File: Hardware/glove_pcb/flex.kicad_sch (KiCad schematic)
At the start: 9 parts

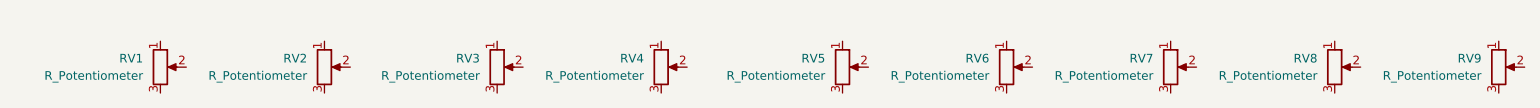
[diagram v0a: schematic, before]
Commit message: More work on motor driver connection
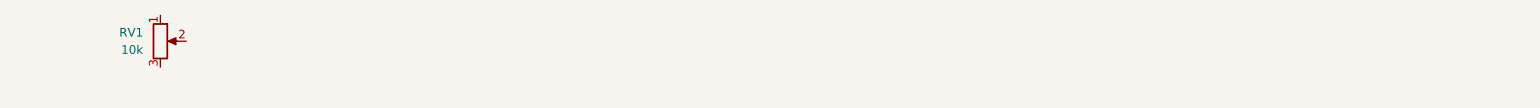
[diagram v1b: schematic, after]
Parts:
- removed RV2, RV3, RV4, RV5, RV6, RV7, RV8, RV9: R_Potentiometer, symbol Device:R_Potentiometer
- RV1: value R_Potentiometer -> 10k
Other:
- moved on the sheet: RV1
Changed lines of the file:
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@@
 (kicad_sch (version 20230121) (generator eeschema)
   (paper "A4")
-  (symbol (lib_id "Device:R_Potentiometer") (at 124.46 45.72 0) (unit 1)
+  (symbol (lib_id "Device:R_Potentiometer") (at 50.8 41.91 0) (unit 1)
     (in_bom yes) (on_board yes) (dnp no) (fields_autoplaced)
-    (property "Reference" "RV4" (at 121.92 44.45 0)
+    (property "Reference" "RV1" (at 48.26 40.64 0)
       (effects (font (size 1.27 1.27)) (justify right))
     )
-    (property "Value" "R_Potentiometer" (at 121.92 46.99 0)
+    (property "Value" "10k" (at 48.26 43.18 0)
       (effects (font (size 1.27 1.27)) (justify right))
     )
-    (property "Footprint" "" (at 124.46 45.72 0)
+    (property "Footprint" "" (at 50.8 41.91 0)
       (effects (font (size 1.27 1.27)) hide)
     )
-    (property "Datasheet" "~" (at 124.46 45.72 0)
-      (effects (font (size 1.27 1.27)) hide)
-    )
-    (pin "1")
-    (pin "2")
-    (pin "3")
-    (instances
-      (project "glove_pcb"
-        (path "/747ff5f3-d342-40b0-8e4e-75b3a3063e75"
-          (reference "RV4") (unit 1)
-        )
-        (path "/747ff5f3-d342-40b0-8e4e-75b3a3063e75/bbbc9975-a050-48bd-8c18-11f2eff17087"
-          (reference "RV4") (unit 1)
-        )
-      )
-    )
-  )
-  (symbol (lib_id "Device:R_Potentiometer") (at 100.33 45.72 0) (unit 1)
-    (in_bom yes) (on_board yes) (dnp no) (fields_autoplaced)
-    (property "Reference" "RV3" (at 97.79 44.45 0)
-      (effects (font (size 1.27 1.27)) (justify right))
-    )
-    (property "Value" "R_Potentiometer" (at 97.79 46.99 0)
-      (effects (font (size 1.27 1.27)) (justify right))
-    )
-    (property "Footprint" "" (at 100.33 45.72 0)
-      (effects (font (size 1.27 1.27)) hide)
-    )
-    (property "Datasheet" "~" (at 100.33 45.72 0)
-      (effects (font (size 1.27 1.27)) hide)
-    )
-    (pin "1")
-    (pin "2")
-    (pin "3")
-    (instances
-      (project "glove_pcb"
-        (path "/747ff5f3-d342-40b0-8e4e-75b3a3063e75"
-          (reference "RV3") (unit 1)
-        )
-        (path "/747ff5f3-d342-40b0-8e4e-75b3a3063e75/bbbc9975-a050-48bd-8c18-11f2eff17087"
-          (reference "RV3") (unit 1)
-        )
-      )
-    )
-  )
-  (symbol (lib_id "Device:R_Potentiometer") (at 223.52 45.72 0) (unit 1)
-    (in_bom yes) (on_board yes) (dnp no) (fields_autoplaced)
-    (property "Reference" "RV8" (at 220.98 44.45 0)
-      (effects (font (size 1.27 1.27)) (justify right))
-    )
-    (property "Value" "R_Potentiometer" (at 220.98 46.99 0)
-      (effects (font (size 1.27 1.27)) (justify right))
-    )
-    (property "Footprint" "" (at 223.52 45.72 0)
-      (effects (font (size 1.27 1.27)) hide)
-    )
-    (property "Datasheet" "~" (at 223.52 45.72 0)
-      (effects (font (size 1.27 1.27)) hide)
-    )
-    (pin "1")
-    (pin "2")
-    (pin "3")
-    (instances
-      (project "glove_pcb"
-        (path "/747ff5f3-d342-40b0-8e4e-75b3a3063e75"
-          (reference "RV8") (unit 1)
-        )
-        (path "/747ff5f3-d342-40b0-8e4e-75b3a3063e75/bbbc9975-a050-48bd-8c18-11f2eff17087"
-          (reference "RV8") (unit 1)
-        )
-      )
-    )
-  )
-  (symbol (lib_id "Device:R_Potentiometer") (at 151.13 45.72 0) (unit 1)
-    (in_bom yes) (on_board yes) (dnp no) (fields_autoplaced)
-    (property "Reference" "RV5" (at 148.59 44.45 0)
-      (effects (font (size 1.27 1.27)) (justify right))
-    )
-    (property "Value" "R_Potentiometer" (at 148.59 46.99 0)
-      (effects (font (size 1.27 1.27)) (justify right))
-    )
-    (property "Footprint" "" (at 151.13 45.72 0)
-      (effects (font (size 1.27 1.27)) hide)
-    )
-    (property "Datasheet" "~" (at 151.13 45.72 0)
-      (effects (font (size 1.27 1.27)) hide)
-    )
-    (pin "1")
-    (pin "2")
-    (pin "3")
-    (instances
-      (project "glove_pcb"
-        (path "/747ff5f3-d342-40b0-8e4e-75b3a3063e75"
-          (reference "RV5") (unit 1)
-        )
-        (path "/747ff5f3-d342-40b0-8e4e-75b3a3063e75/bbbc9975-a050-48bd-8c18-11f2eff17087"
-          (reference "RV5") (unit 1)
-        )
-      )
-    )
-  )
-  (symbol (lib_id "Device:R_Potentiometer") (at 175.26 45.72 0) (unit 1)
-    (in_bom yes) (on_board yes) (dnp no) (fields_autoplaced)
-    (property "Reference" "RV6" (at 172.72 44.45 0)
-      (effects (font (size 1.27 1.27)) (justify right))
-    )
-    (property "Value" "R_Potentiometer" (at 172.72 46.99 0)
-      (effects (font (size 1.27 1.27)) (justify right))
-    )
-    (property "Footprint" "" (at 175.26 45.72 0)
-      (effects (font (size 1.27 1.27)) hide)
-    )
-    (property "Datasheet" "~" (at 175.26 45.72 0)
-      (effects (font (size 1.27 1.27)) hide)
-    )
-    (pin "1")
-    (pin "2")
-    (pin "3")
-    (instances
-      (project "glove_pcb"
-        (path "/747ff5f3-d342-40b0-8e4e-75b3a3063e75"
-          (reference "RV6") (unit 1)
-        )
-        (path "/747ff5f3-d342-40b0-8e4e-75b3a3063e75/bbbc9975-a050-48bd-8c18-11f2eff17087"
-          (reference "RV6") (unit 1)
-        )
-      )
-    )
-  )
-  (symbol (lib_id "Device:R_Potentiometer") (at 50.8 45.72 0) (unit 1)
-    (in_bom yes) (on_board yes) (dnp no) (fields_autoplaced)
-    (property "Reference" "RV1" (at 48.26 44.45 0)
-      (effects (font (size 1.27 1.27)) (justify right))
-    )
-    (property "Value" "R_Potentiometer" (at 48.26 46.99 0)
-      (effects (font (size 1.27 1.27)) (justify right))
-    )
-    (property "Footprint" "" (at 50.8 45.72 0)
-      (effects (font (size 1.27 1.27)) hide)
-    )
-    (property "Datasheet" "~" (at 50.8 45.72 0)
+    (property "Datasheet" "~" (at 50.8 41.91 0)
       (effects (font (size 1.27 1.27)) hide)
     )
@@
         )
       )
-    )
-  )
-  (symbol (lib_id "Device:R_Potentiometer") (at 74.93 45.72 0) (unit 1)
-    (in_bom yes) (on_board yes) (dnp no) (fields_autoplaced)
-    (property "Reference" "RV2" (at 72.39 44.45 0)
-      (effects (font (size 1.27 1.27)) (justify right))
-    )
-    (property "Value" "R_Potentiometer" (at 72.39 46.99 0)
-      (effects (font (size 1.27 1.27)) (justify right))
-    )
-    (property "Footprint" "" (at 74.93 45.72 0)
-      (effects (font (size 1.27 1.27)) hide)
-    )
-    (property "Datasheet" "~" (at 74.93 45.72 0)
-      (effects (font (size 1.27 1.27)) hide)
-    )
-    (pin "1")
-    (pin "2")
-    (pin "3")
-    (instances
-      (project "glove_pcb"
-        (path "/747ff5f3-d342-40b0-8e4e-75b3a3063e75"
-          (reference "RV2") (unit 1)
-        )
-        (path "/747ff5f3-d342-40b0-8e4e-75b3a3063e75/bbbc9975-a050-48bd-8c18-11f2eff17087"
-          (reference "RV2") (unit 1)
-        )
-      )
-    )
-  )
-  (symbol (lib_id "Device:R_Potentiometer") (at 199.39 45.72 0) (unit 1)
-    (in_bom yes) (on_board yes) (dnp no) (fields_autoplaced)
-    (property "Reference" "RV7" (at 196.85 44.45 0)
-      (effects (font (size 1.27 1.27)) (justify right))
-    )
-    (property "Value" "R_Potentiometer" (at 196.85 46.99 0)
-      (effects (font (size 1.27 1.27)) (justify right))
-    )
-    (property "Footprint" "" (at 199.39 45.72 0)
-      (effects (font (size 1.27 1.27)) hide)
-    )
-    (property "Datasheet" "~" (at 199.39 45.72 0)
-      (effects (font (size 1.27 1.27)) hide)
-    )
-    (pin "1")
-    (pin "2")
-    (pin "3")
-    (instances
-      (project "glove_pcb"
-        (path "/747ff5f3-d342-40b0-8e4e-75b3a3063e75"
-          (reference "RV7") (unit 1)
-        )
-        (path "/747ff5f3-d342-40b0-8e4e-75b3a3063e75/bbbc9975-a050-48bd-8c18-11f2eff17087"
-          (reference "RV7") (unit 1)
-        )
-      )
-    )
-  )
-  (symbol (lib_id "Device:R_Potentiometer") (at 247.65 45.72 0) (unit 1)
-    (in_bom yes) (on_board yes) (dnp no) (fields_autoplaced)
-    (property "Reference" "RV9" (at 245.11 44.45 0)
-      (effects (font (size 1.27 1.27)) (justify right))
-    )
-    (property "Value" "R_Potentiometer" (at 245.11 46.99 0)
-      (effects (font (size 1.27 1.27)) (justify right))
-    )
-    (property "Footprint" "" (at 247.65 45.72 0)
-      (effects (font (size 1.27 1.27)) hide)
-    )
-    (property "Datasheet" "~" (at 247.65 45.72 0)
-      (effects (font (size 1.27 1.27)) hide)
-    )
-    (pin "1")
-    (pin "2")
-    (pin "3")
-    (instances
-      (project "glove_pcb"
-        (path "/747ff5f3-d342-40b0-8e4e-75b3a3063e75"
-          (reference "RV9") (unit 1)
-        )
-        (path "/747ff5f3-d342-40b0-8e4e-75b3a3063e75/bbbc9975-a050-48bd-8c18-11f2eff17087"
-          (reference "RV9") (unit 1)
-        )
-      )
